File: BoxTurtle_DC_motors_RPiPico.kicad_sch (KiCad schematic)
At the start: 40 parts, among them J1 Power input, J10 DC motor 1, J11 DC motor 2, J12 DC motor 3, J13 DC motor 4, J14 Screw_Terminal_01x02, J15 CAN, J2 Power input, J3 Power output, J4 Power output, J5 AMS1117 module, J6 DRV8837 module left, J7 DRV8837 module right, J8 DRV8837 module left, J9 DRV8837 module right, SW1 Conn_01x03, SW10 Conn_01x03, SW11 Conn_01x03, SW12 Conn_01x03, SW13 K3-1204D, SW2 Conn_01x03, SW3 Conn_01x03, SW4 Conn_01x03, SW5 Conn_01x03, SW6 Conn_01x03, SW7 Conn_01x03, SW8 Conn_01x03, SW9 Conn_01x03, U1 Raspberry Pi Pico, U2 Black Pill STM32F401

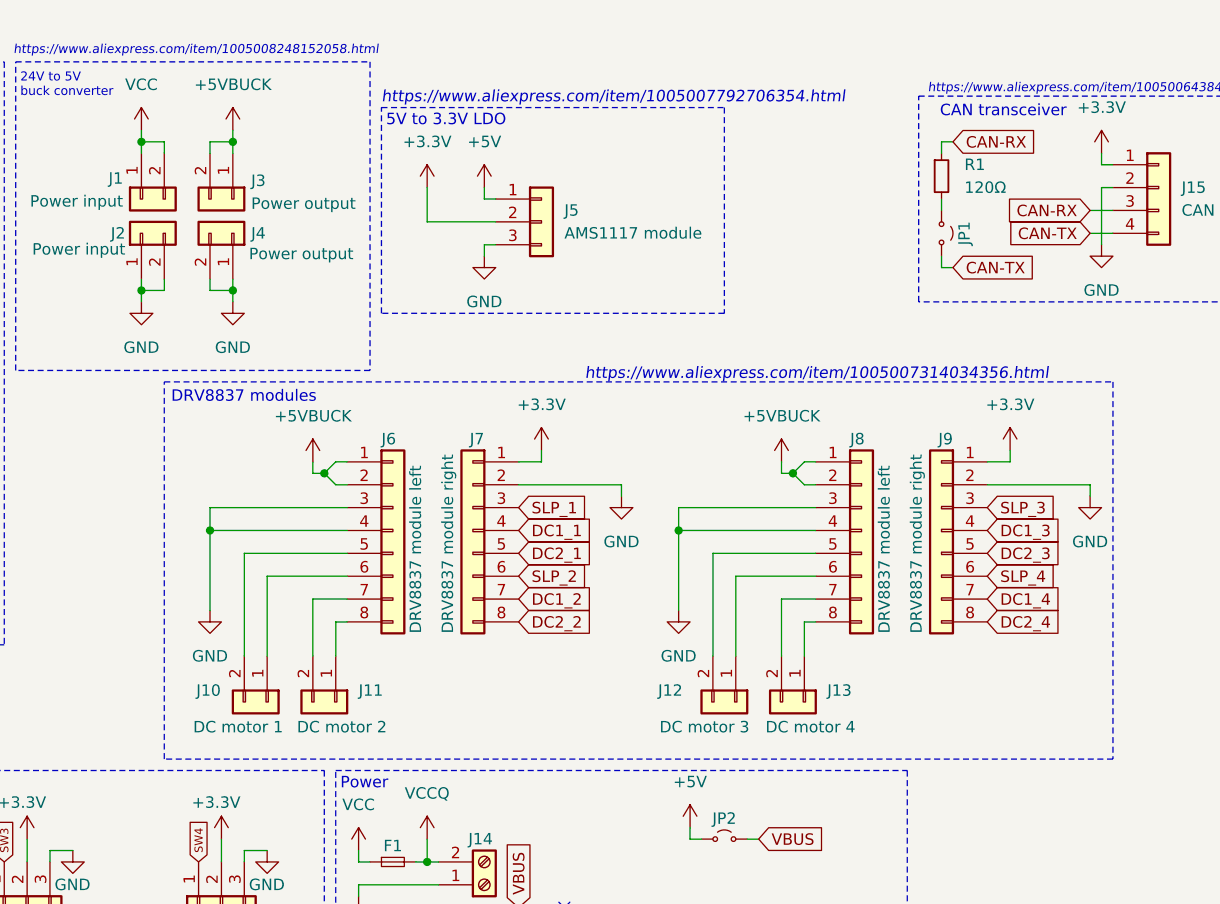
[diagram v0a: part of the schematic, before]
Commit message: Revision 2.6.4
Will update the Gerber files later
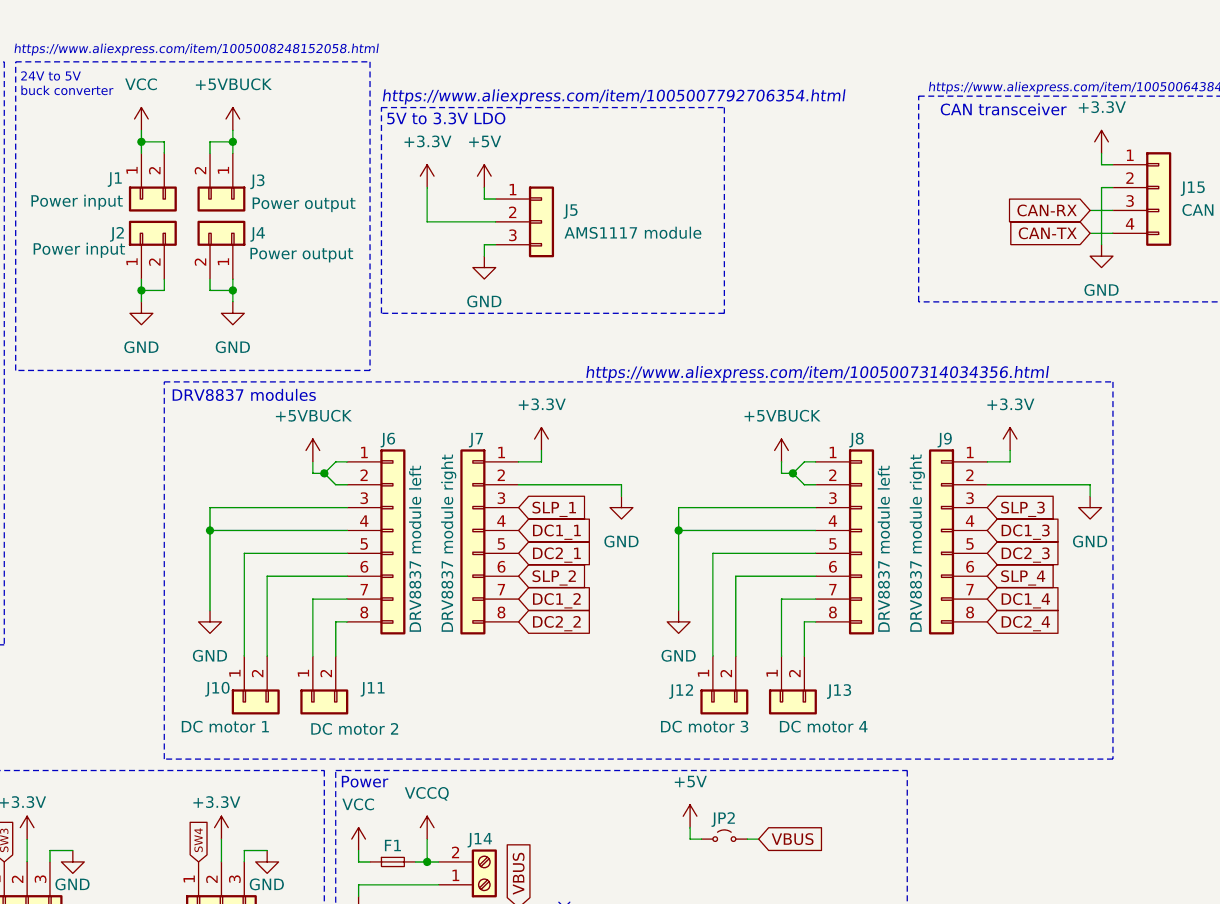
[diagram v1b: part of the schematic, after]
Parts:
- removed JP1: Jumper_2_Small_Open, Connector_PinHeader_2.54mm:PinHeader_1x02_P2.54mm_Vertical, symbol Jumper:Jumper_2_Small_Open
- removed R1: 120Ω, Resistor_THT:R_Axial_DIN0207_L6.3mm_D2.5mm_P10.16mm_Horizontal, symbol Device:R_Small
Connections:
- net at J6.5 (Pin_5): now also J10.1 (Pin_1); no longer J10.2 (Pin_2)
- net at J6.6 (Pin_6): now also J10.2 (Pin_2); no longer J10.1 (Pin_1)
- net at J6.7 (Pin_7): now also J11.1 (Pin_1); no longer J11.2 (Pin_2)
- net at J6.8 (Pin_8): now also J11.2 (Pin_2); no longer J11.1 (Pin_1)
- net at J8.5 (Pin_5): now also J12.1 (Pin_1); no longer J12.2 (Pin_2)
- net at J8.6 (Pin_6): now also J12.2 (Pin_2); no longer J12.1 (Pin_1)
- net at J8.7 (Pin_7): now also J13.1 (Pin_1); no longer J13.2 (Pin_2)
- net at J8.8 (Pin_8): now also J13.2 (Pin_2); no longer J13.1 (Pin_1)
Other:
- moved on the sheet: J10, J11, J12, J13
